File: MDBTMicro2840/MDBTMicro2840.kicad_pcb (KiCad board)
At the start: 2 copper layers, 4 parts, among them J1 Conn_01x04, J2 USB_C_Receptacle_USB2.0, U1 MDBT50Q-x1MV2, U2 ProMicro

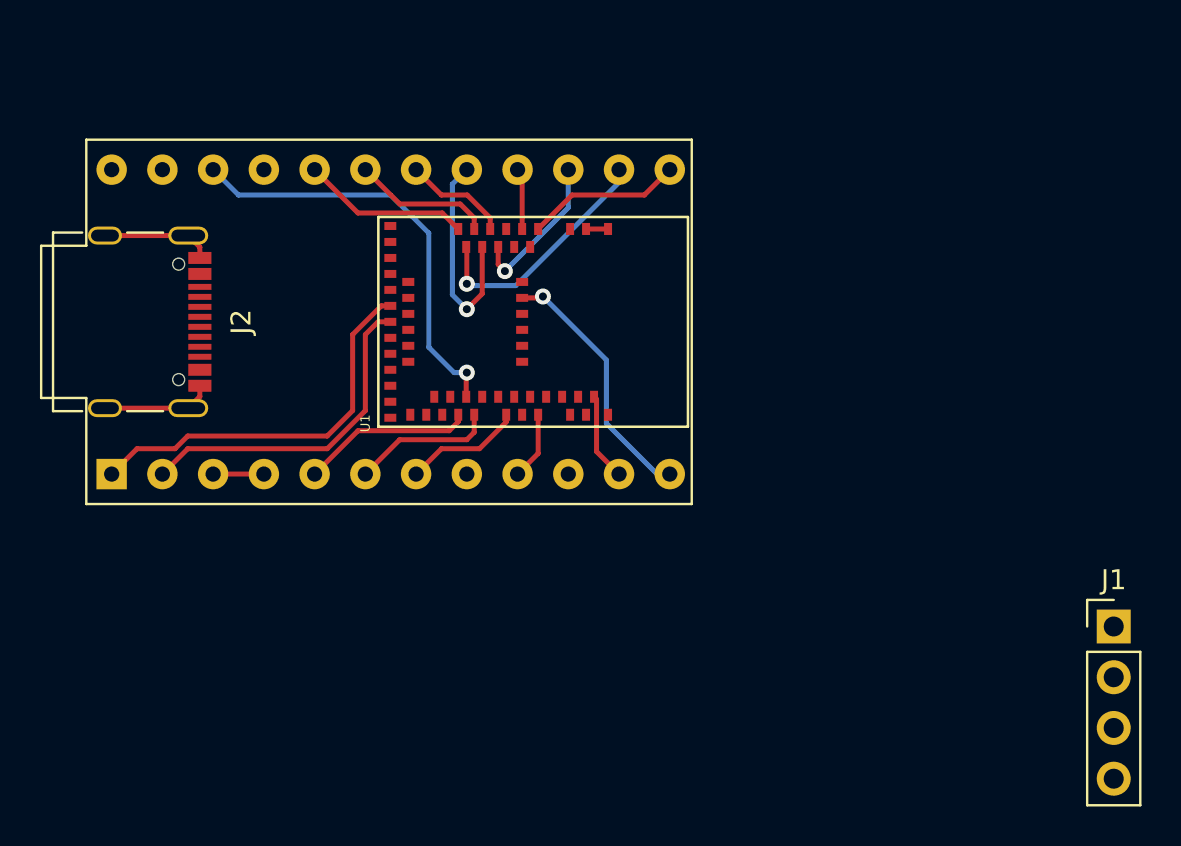
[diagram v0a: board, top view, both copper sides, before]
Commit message: Update sch
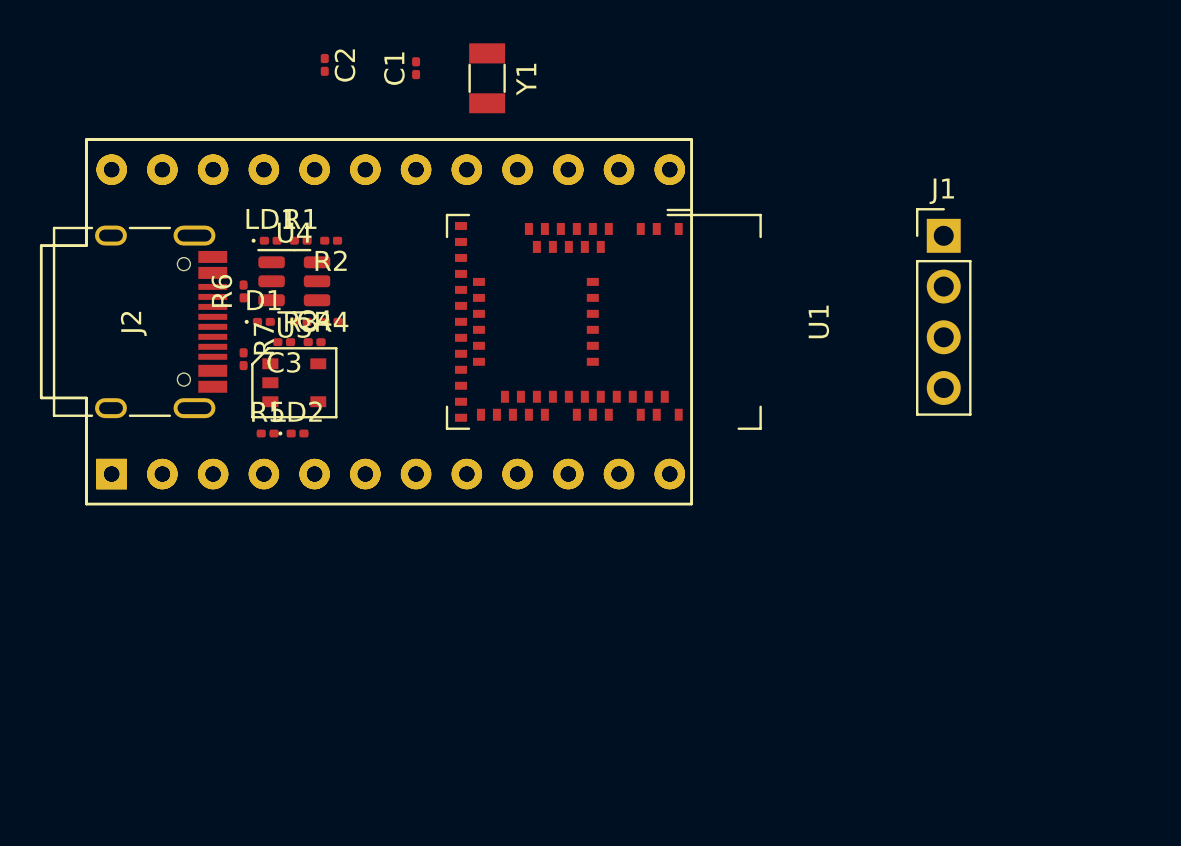
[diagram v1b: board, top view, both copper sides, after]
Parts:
- added C1: 12pF, Capacitor_SMD:C_0201_0603Metric, F.Cu at (142.2, 81.3)
- added C2: 12pF, Capacitor_SMD:C_0201_0603Metric, F.Cu at (137.7, 81.1)
- added C3: 10uF, Capacitor_SMD:C_0201_0603Metric, F.Cu at (135.6, 95.0)
- added C4: 10uF, Capacitor_SMD:C_0201_0603Metric, F.Cu at (137.2, 95.0)
- added D1: 1N5819, Diode_SMD:D_0201_0603Metric, F.Cu at (134.6, 94.0)
- added LD1: RED, LED_SMD:LED_0201_0603Metric, F.Cu at (135.0, 89.9)
- added LD2: BLUE, LED_SMD:LED_0201_0603Metric, F.Cu at (136.3, 99.6)
- added R1: 1k, Resistor_SMD:R_0201_0603Metric, F.Cu at (136.5, 89.9)
- added R2: Rprog, Resistor_SMD:R_0201_0603Metric, F.Cu at (138.0, 89.9)
- added R3: 820k, Resistor_SMD:R_0201_0603Metric, F.Cu at (136.5, 94.0)
- added R4: 2M, Resistor_SMD:R_0201_0603Metric, F.Cu at (138.0, 94.0)
- added R5: 1k, Resistor_SMD:R_0201_0603Metric, F.Cu at (134.8, 99.6)
- added R6: 5.1k, Resistor_SMD:R_0201_0603Metric, F.Cu at (133.6, 92.5)
- added R7: 5.1k, Resistor_SMD:R_0201_0603Metric, F.Cu at (133.6, 95.8)
- added U2: ProMicro, MDBTMicro_library:ProMicro, F.Cu at (127.0, 101.6)
- added U3: XC6220B331MR-G, MDBTMicro_library:SOT-25-5, F.Cu at (136.1, 97.0)
- added U4: TP4057, Package_TO_SOT_SMD:SOT-23-6, F.Cu at (136.1, 91.9)
- added Y1: 32.768kHz, Crystal:Crystal_SMD_3215-2Pin_3.2x1.5mm, F.Cu at (145.8, 81.8)
- J1: value Conn_01x04 -> SWD
- J2: footprint Connector_USB:USB_C_Receptacle_Palconn_UTC16-G -> Connector_USB:USB_C_Receptacle_HRO_TYPE-C-31-M-12
- U1: footprint MDBTMicro_library:MDBT50Q -> RF_Module:Raytac_MDBT50Q
- moved J1 21.3 mm to (168.7, 89.7)
- moved U1 3.54 mm to (151.6, 94.0)
- moved J2 0.89 mm to (128.0, 94.0)
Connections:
- net /RESET renamed RESET
- net /SWDCLK renamed SWCLK
- net /SWDIO renamed SWDIO
- net /USB_D+ renamed USB_D+
- net /USB_D- renamed USB_D-
- net /VBUS renamed VBUS
- J1 pad 1: VDD -> nRF_VDD
- J2 pad A5: unconnected-(J2-PadA5) -> Net-(J2-PadA5)
- J2 pad B5: unconnected-(J2-PadB5) -> Net-(J2-PadB5)
- J2 pad S1: GND -> unconnected-(J2-PadS1)
- U1 pad 15: unconnected-(U1-Pad15) -> GND
- U1 pad 17: unconnected-(U1-Pad17) -> Net-(U1-Pad17)
- U1 pad 18: unconnected-(U1-Pad18) -> Net-(U1-Pad18)
- U1 pad 20: unconnected-(U1-Pad20) -> BATTERT_PIN
- U1 pad 28: VDD -> nRF_VDD
- U1 pad 3: unconnected-(U1-Pad3) -> LED_PIN
- U1 pad 30: unconnected-(U1-Pad30) -> nRF_VDD
- U1 pad 33: unconnected-(U1-Pad33) -> GND
- U1 pad 55: unconnected-(U1-Pad55) -> GND
- U2 pad 13: unconnected-(U2-Pad13) -> VBAT
- U2 pad 14: unconnected-(U2-Pad14) -> GND
- U2 pad 16: unconnected-(U2-Pad16) -> nRF_VDD
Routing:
- net RESET: track 21.5 -> 0.00 mm, vias 1 -> 0
- net /P0.06: track 19.7 -> 0.00 mm
- net /P0.08: track 16.8 -> 0.00 mm
- net GND: track 14.7 -> 0.00 mm
- net /P1.06: track 13.0 -> 0.00 mm, vias 1 -> 0
- net /P0.28: track 12.3 -> 0.00 mm, vias 1 -> 0
- net /P0.02: track 11.0 -> 0.00 mm, vias 1 -> 0
- net /P0.15: track 8.63 -> 0.00 mm
- net /P0.30: track 8.42 -> 0.00 mm
- net /P1.11: track 7.82 -> 0.00 mm
- net /P0.03: track 7.74 -> 0.00 mm, vias 1 -> 0
- net /P0.17: track 7.20 -> 0.00 mm
- net /P0.31: track 7.00 -> 0.00 mm
- net /P0.20: track 5.95 -> 0.00 mm
- net /P0.29: track 5.26 -> 0.00 mm
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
